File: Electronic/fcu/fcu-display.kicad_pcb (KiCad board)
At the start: 2 copper layers, 34 parts, among them U101 Connector-FPC-50pins

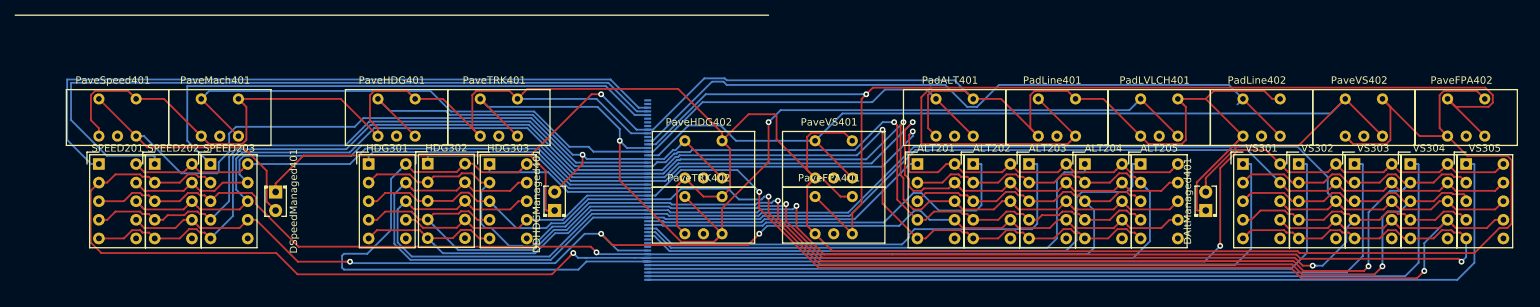
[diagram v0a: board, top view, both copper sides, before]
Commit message: Update fcu schemas and libraries
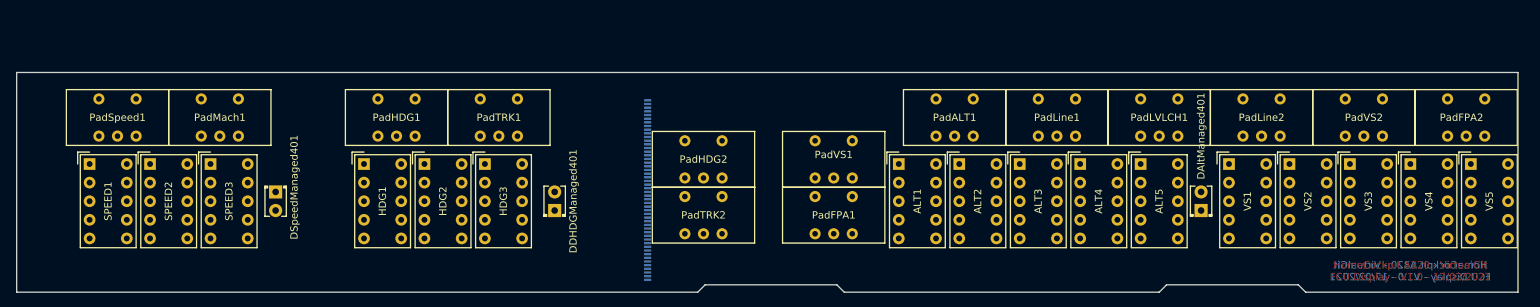
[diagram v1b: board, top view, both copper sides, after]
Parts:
- removed ALT201, ALT202, ALT203, ALT204, ALT205, HDG301, HDG302, HDG303, SPEED201, SPEED202, SPEED203, VS301, VS302, VS303, VS304, VS305: HDSP-7403, Display_7Segment:HDSP-7401
- added ALT1: HDSP-7401, Display_7Segment:HDSP-7401, F.Cu at (171.4, 63.5)
- added ALT2: HDSP-7401, Display_7Segment:HDSP-7401, F.Cu at (179.7, 63.5)
- added ALT3: HDSP-7401, Display_7Segment:HDSP-7401, F.Cu at (188.0, 63.5)
- added ALT4: HDSP-7401, Display_7Segment:HDSP-7401, F.Cu at (196.2, 63.5)
- added ALT5: HDSP-7401, Display_7Segment:HDSP-7401, F.Cu at (204.5, 63.5)
- added HDG1: HDSP-7401, Display_7Segment:HDSP-7401, F.Cu at (98.4, 63.5)
- added HDG2: HDSP-7401, Display_7Segment:HDSP-7401, F.Cu at (106.7, 63.5)
- added HDG3: HDSP-7401, Display_7Segment:HDSP-7401, F.Cu at (114.9, 63.5)
- added SPEED1: HDSP-7401, Display_7Segment:HDSP-7401, F.Cu at (61.0, 63.5)
- added SPEED2: HDSP-7401, Display_7Segment:HDSP-7401, F.Cu at (69.2, 63.5)
- added SPEED3: HDSP-7401, Display_7Segment:HDSP-7401, F.Cu at (77.5, 63.5)
- added VS1: HDSP-7401, Display_7Segment:HDSP-7401, F.Cu at (216.5, 63.5)
- added VS2: HDSP-7401, Display_7Segment:HDSP-7401, F.Cu at (224.8, 63.5)
- added VS3: HDSP-7401, Display_7Segment:HDSP-7401, F.Cu at (233.0, 63.5)
- added VS4: HDSP-7401, Display_7Segment:HDSP-7401, F.Cu at (241.3, 63.5)
- added VS5: HDSP-7401, Display_7Segment:HDSP-7401, F.Cu at (249.6, 63.5)
- moved DAltManaged401 0.64 mm to (212.7, 69.8)
- renumbered PadALT401 to PadALT1, PaveFPA401 to PadFPA1, PaveFPA402 to PadFPA2, PaveHDG401 to PadHDG1, PaveHDG402 to PadHDG2, PadLVLCH401 to PadLVLCH1, PadLine401 to PadLine1, PadLine402 to PadLine2, PaveMach401 to PadMach1, PaveSpeed401 to PadSpeed1, PaveTRK401 to PadTRK1, PaveTRK402 to PadTRK2, PaveVS401 to PadVS1, PaveVS402 to PadVS2
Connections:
- PadSpeed1 pad 3: Dr3SegA -> Net-(PadSpeed1-Pad3)
- PadSpeed1 pad 6: Dr3SegA -> Net-(PadSpeed1-Pad3)
- U101 pad 1: hdgVsDig3 -> Net-(U101-Pad1)
- U101 pad 10: Dr3Dig5 -> Dr3Dig0
- U101 pad 11: Dr3Dig6 -> Dr3SegDP
- U101 pad 12: Dr3Dig7 -> Dr3SegG
- U101 pad 13: speedAltDig3 -> Dr3SegF
- U101 pad 14: speedAltDig4 -> Dr3SegE
- U101 pad 15: speedAltDig5 -> Dr3SegD
- U101 pad 16: speedAltDig6 -> Dr3SegC
- U101 pad 17: speedAltDig7 -> Dr3SegB
- U101 pad 18: hdgVsB -> Dr3SegA
- U101 pad 19: hdgVsC -> speedAltE
- U101 pad 2: hdgVsDig4 -> Net-(U101-Pad2)
- U101 pad 20: hdgVsD -> speedAltD
- U101 pad 21: hdgVsE -> speedAltC
- U101 pad 22: hdgVsF -> speedAltB
- U101 pad 23: hdgVsG -> speedAltA
- U101 pad 24: hdgVsDP -> hdgVsDig2
- U101 pad 25: hdgVsDig0 -> hdgVsDig1
- U101 pad 26: hdgVsDig1 -> hdgVsDig0
- U101 pad 27: hdgVsDig2 -> hdgVsDP
- U101 pad 28: speedAltA -> hdgVsG
- U101 pad 29: speedAltB -> hdgVsF
- U101 pad 3: hdgVsDig5 -> speedAltDig2
- U101 pad 30: speedAltC -> hdgVsE
- U101 pad 31: speedAltD -> hdgVsD
- U101 pad 32: speedAltE -> hdgVsC
- U101 pad 33: Dr3SegA -> hdgVsB
- U101 pad 34: Dr3SegB -> speedAltDig7
- U101 pad 35: Dr3SegC -> speedAltDig6
- U101 pad 36: Dr3SegD -> speedAltDig5
- U101 pad 37: Dr3SegE -> speedAltDig4
- U101 pad 38: Dr3SegF -> speedAltDig3
- U101 pad 39: Dr3SegG -> Dr3Dig7
- U101 pad 4: hdgVsDig6 -> speedAltDig1
- U101 pad 40: Dr3SegDP -> Dr3Dig6
- U101 pad 41: Dr3Dig0 -> Dr3Dig5
- U101 pad 42: Dr3Dig1 -> speedAltDP
- U101 pad 43: Dr3Dig2 -> speedAltG
- U101 pad 44: Dr3Dig3 -> speedAltF
- U101 pad 45: Dr3Dig4 -> hdgVsA
- U101 pad 46: speedAltDig0 -> hdgVsDig7
- U101 pad 47: speedAltDig1 -> hdgVsDig6
- U101 pad 48: speedAltDig2 -> hdgVsDig5
- U101 pad 49: Net-(U101-Pad49) -> hdgVsDig4
- U101 pad 5: hdgVsDig7 -> speedAltDig0
- U101 pad 50: Net-(U101-Pad50) -> hdgVsDig3
- U101 pad 6: hdgVsA -> Dr3Dig4
- U101 pad 7: speedAltF -> Dr3Dig3
- U101 pad 8: speedAltG -> Dr3Dig2
- U101 pad 9: speedAltDP -> Dr3Dig1
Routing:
- net Dr3Dig0: track 369.3 -> 0.00 mm
- net speedAltF: track 218.3 -> 0.00 mm, vias 1 -> 0
- net hdgVsA: track 214.8 -> 0.00 mm, vias 1 -> 0
- net Dr3Dig1: track 214.1 -> 0.00 mm, vias 1 -> 0
- net hdgVsD: track 205.8 -> 0.00 mm, vias 2 -> 0
- net hdgVsF: track 204.3 -> 0.00 mm, vias 2 -> 0
- net Dr3SegF: track 198.4 -> 0.00 mm, vias 1 -> 0
- net hdgVsC: track 198.4 -> 0.00 mm
- net hdgVsG: track 197.0 -> 0.00 mm, vias 2 -> 0
- net hdgVsDP: track 194.1 -> 0.00 mm, vias 2 -> 0
- net hdgVsE: track 192.3 -> 0.00 mm, vias 2 -> 0
- net hdgVsB: track 191.7 -> 0.00 mm
- net speedAltG: track 184.0 -> 0.00 mm, vias 1 -> 0
- net speedAltD: track 176.2 -> 0.00 mm, vias 1 -> 0
- net speedAltC: track 175.0 -> 0.00 mm, vias 1 -> 0
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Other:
- board outline added: 205 x 30 mm
- board text added: "HomeCockpit A320 - VirtualGit FCU Display - V1.0 - 17/02/2021"
